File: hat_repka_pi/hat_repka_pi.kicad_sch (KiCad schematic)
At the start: 3 parts, among them Q1 BD233

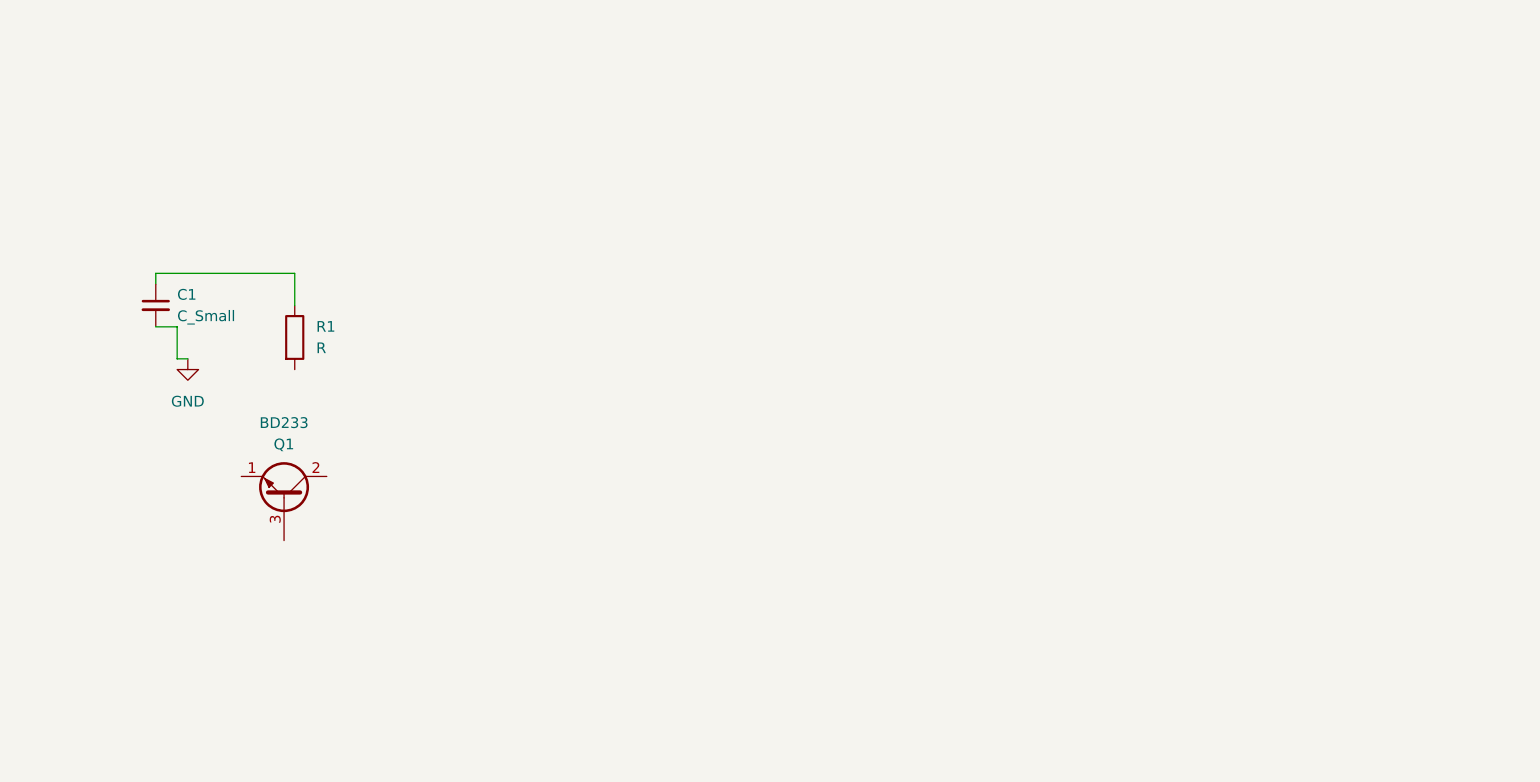
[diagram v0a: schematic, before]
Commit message: Добавлены основные компоненты на плату
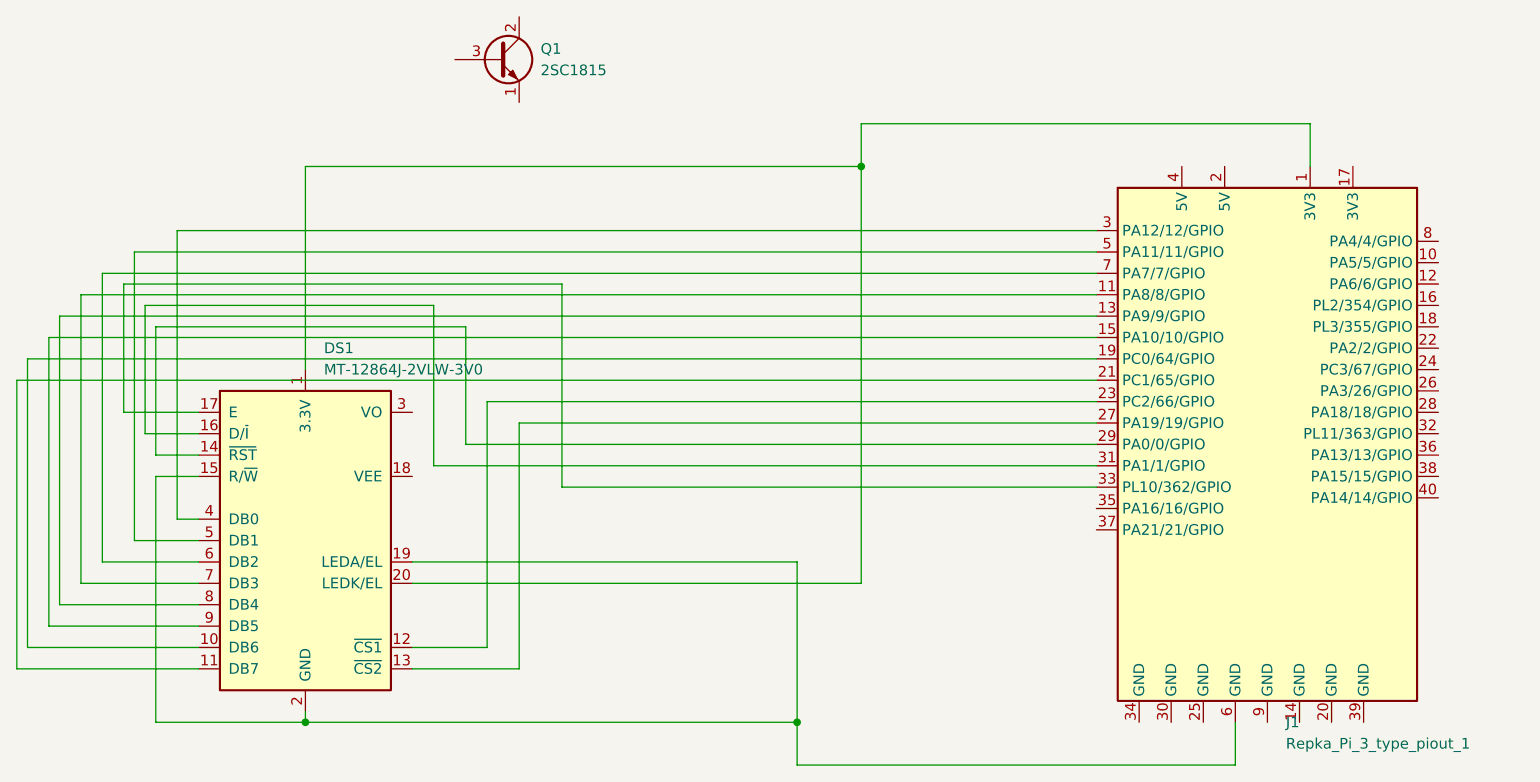
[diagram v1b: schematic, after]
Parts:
- removed C1: C_Small, symbol Device:C_Small
- removed Q1: BD233, Package_TO_SOT_THT:TO-126-3_Vertical, symbol Transistor_BJT:BD233
- removed R1: R, symbol Device:R
- added DS1: MT-12864J-2VLW-3V0, Display:MT-12864J-2VLW-3V0, symbol Melt:MT-12864J-2VLW-3V0
- added J1: Repka_Pi_3_type_piout_1, symbol Repka-Pi3:Repka_Pi_3_type_piout_1
- added Q1: 2SC1815, Package_TO_SOT_THT:TO-92_Inline, symbol Transistor_BJT:2SC1815
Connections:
- new net: DS1.1 (3.3V), DS1.20 (LEDK/EL), J1.1 (3V3)
- new net: DS1.10 (DB6), J1.19 (PC0/64/GPIO)
- new net: DS1.11 (DB7), J1.21 (PC1/65/GPIO)
- new net: DS1.12 (~{CS1}), J1.23 (PC2/66/GPIO)
- new net: DS1.13 (~{CS2}), J1.27 (PA19/19/GPIO)
- new net: DS1.14 (~{RST}), J1.29 (PA0/0/GPIO)
- new net: DS1.15 (R/~{W}), DS1.19 (LEDA/EL), DS1.2 (GND), J1.6 (GND)
- new net: DS1.16 (D/~{I}), J1.31 (PA1/1/GPIO)
- new net: DS1.17 (E), J1.33 (PL10/362/GPIO)
- new net: DS1.4 (DB0), J1.3 (PA12/12/GPIO)
- new net: DS1.5 (DB1), J1.5 (PA11/11/GPIO)
- new net: DS1.6 (DB2), J1.7 (PA7/7/GPIO)
- new net: DS1.7 (DB3), J1.11 (PA8/8/GPIO)
- new net: DS1.8 (DB4), J1.13 (PA9/9/GPIO)
- new net: DS1.9 (DB5), J1.15 (PA10/10/GPIO)
